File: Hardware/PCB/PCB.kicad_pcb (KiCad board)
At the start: 2 copper layers, 50.2 x 30.8 mm, 3 parts, among them P1 USB_C_Plug_USB2.0, U1 ESP32-H2-MINI-1, U3 AMS1117-3.3

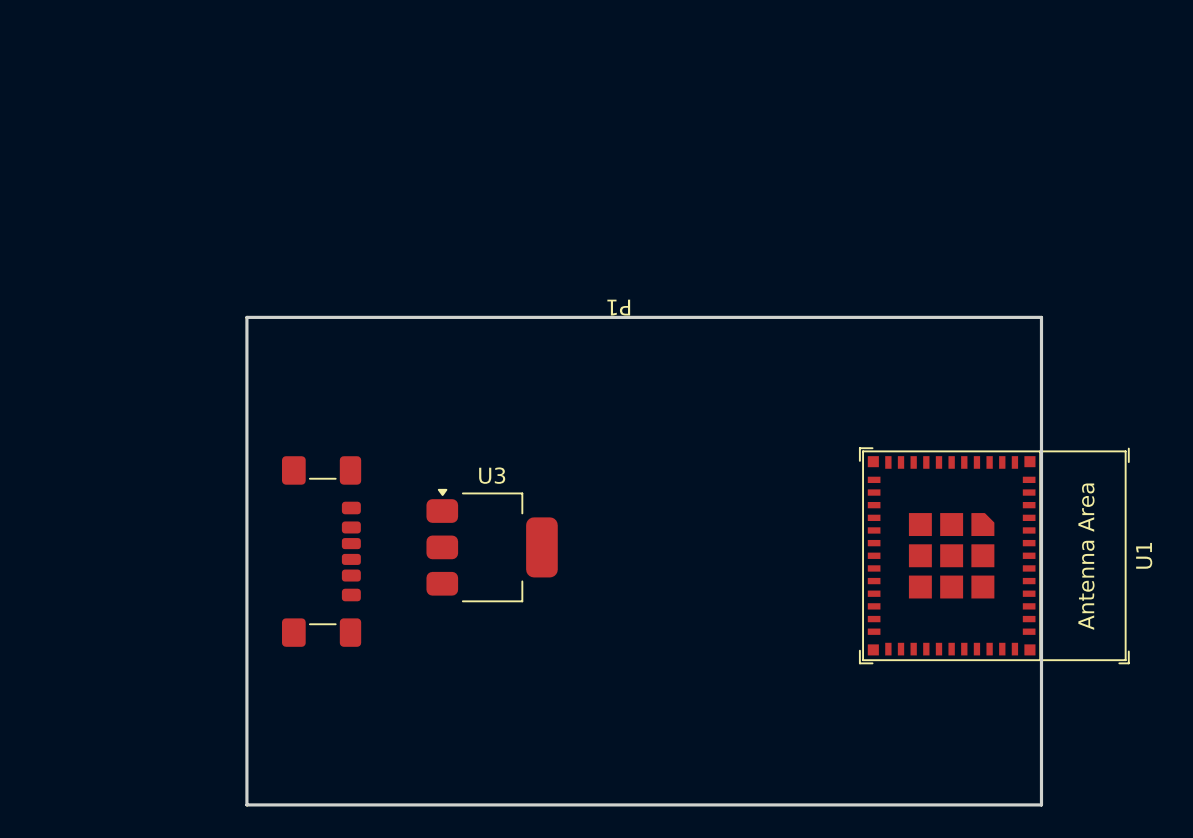
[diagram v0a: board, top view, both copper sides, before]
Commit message: First pass at full layout
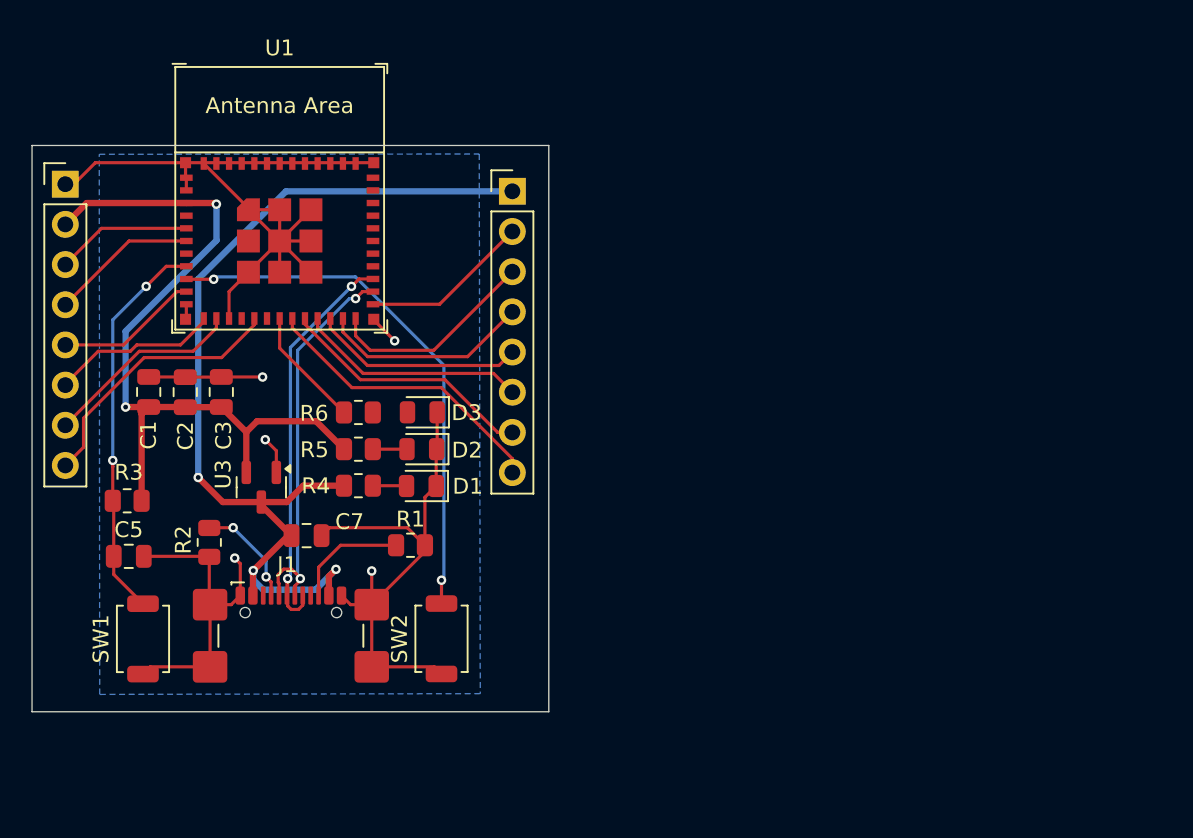
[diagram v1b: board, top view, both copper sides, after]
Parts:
- removed P1: USB_C_Plug_USB2.0, Connector_USB:USB_C_Receptacle_GCT_USB4135-GF-A_6P_TopMnt_Horizontal
- added C1: 10µ, Capacitor_SMD:C_0805_2012Metric, F.Cu at (97.3, 54.6)
- added C2: 1µF, Capacitor_SMD:C_0805_2012Metric, F.Cu at (99.6, 54.6)
- added C3: 0.1µ, Capacitor_SMD:C_0805_2012Metric, F.Cu at (101.9, 54.6)
- added C5: 1µ, Capacitor_SMD:C_0805_2012Metric, F.Cu at (96.0, 65.0)
- added C7: 1µF, Capacitor_SMD:C_0805_2012Metric, F.Cu at (107.3, 63.7)
- added D1: LED, LED_SMD:LED_0805_2012Metric, F.Cu at (114.5, 60.6)
- added D2: LED, LED_SMD:LED_0805_2012Metric, F.Cu at (114.6, 58.2)
- added D3: LED, LED_SMD:LED_0805_2012Metric, F.Cu at (114.6, 55.9)
- added J1: USB_C_Receptacle_USB2.0_14P, Connector_USB:USB_C_Receptacle_GCT_USB4110, F.Cu at (106.3, 71.2)
- added J2: Conn_01x08_Pin, Connector_PinHeader_2.54mm:PinHeader_1x08_P2.54mm_Vertical, F.Cu at (92.0, 41.5)
- added J3: Conn_01x8_Pin, Connector_PinHeader_2.54mm:PinHeader_1x08_P2.54mm_Vertical, F.Cu at (120.3, 41.9)
- added R1: 5.1K, Resistor_SMD:R_0805_2012Metric, F.Cu at (113.8, 64.3)
- added R2: 5.1K, Resistor_SMD:R_0805_2012Metric, F.Cu at (101.1, 64.1)
- added R3: 10K, Resistor_SMD:R_0805_2012Metric, F.Cu at (95.9, 61.5)
- added R4: 5.1K, Resistor_SMD:R_0805_2012Metric, F.Cu at (110.6, 60.5)
- added R5: 5.1K, Resistor_SMD:R_0805_2012Metric, F.Cu at (110.6, 58.2)
- added R6: 5.1K, Resistor_SMD:R_0805_2012Metric, F.Cu at (110.6, 55.9)
- added SW1: SW_Push, Button_Switch_SMD:SW_SPST_TS-1088-xR025, F.Cu at (96.9, 70.2)
- added SW2: SW_Push, Button_Switch_SMD:SW_SPST_TS-1088-xR025, F.Cu at (115.8, 70.2)
- U3: value AMS1117-3.3 -> MCP1700x-330xxTT; footprint Package_TO_SOT_SMD:SOT-223-3_TabPin2 -> Package_TO_SOT_SMD:SOT-23
- moved U1 50.5 mm to (105.6, 42.4), turned to 0 degrees
- moved U3 15.1 mm to (104.4, 60.6), turned to -90 degrees
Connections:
- net Net-(U1-3V3) renamed +3.3V
- U1 pad 10: unconnected-(U1-GPIO1/FSPICS0/ADC1_CH0-Pad10) -> GPIO1
- U1 pad 12: unconnected-(U1-GPIO13/XTAL_32K_P-Pad12) -> GPIO13
- U1 pad 13: unconnected-(U1-GPIO14/XTAL_32K_N-Pad13) -> GPIO14
- U1 pad 16: unconnected-(U1-GPIO12-Pad16) -> GPIO12
- U1 pad 18: unconnected-(U1-GPIO4/FSPICLK/ADC1_CH3/MTCK-Pad18) -> GPIO4
- U1 pad 19: unconnected-(U1-GPIO5/FSPID/ADC1_CH4/MTDI-Pad19) -> GPIO5
- U1 pad 20: unconnected-(U1-GPIO10/ZCD0-Pad20) -> GPIO10
- U1 pad 21: unconnected-(U1-GPIO11/ZCD1-Pad21) -> GPIO11
- U1 pad 22: unconnected-(U1-GPIO8-Pad22) -> GPIO8
- U1 pad 23: unconnected-(U1-GPIO9-Pad23) -> GPIO9
- U1 pad 24: unconnected-(U1-GPIO22-Pad24) -> GPIO22
- U1 pad 25: unconnected-(U1-GPIO25/FSPICS3-Pad25) -> GPIO25
- U1 pad 26: /USB_D- -> USB_D-
- U1 pad 27: /USB_D+ -> USB_D+
- U1 pad 30: unconnected-(U1-GPIO23/FSPICS1/U0RXD-Pad30) -> GPIO23
- U1 pad 31: unconnected-(U1-GPIO24/FSPICS2/U0TXD-Pad31) -> GPIO24
- U1 pad 5: unconnected-(U1-GPIO2/FSPIWP/ADC1_CH1/MTMS-Pad5) -> GPIO2
- U1 pad 6: unconnected-(U1-GPIO3/FSPIHD/ADC1_CH2/MTDO-Pad6) -> GPIO3
- U1 pad 8: unconnected-(U1-EN-Pad8) -> EN
- U1 pad 9: unconnected-(U1-GPIO0/FSPIQ-Pad9) -> BOOT
- U3 pad 3: Net-(U3-VI) -> +5V
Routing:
- net GND: track 0.00 -> 114.8 mm, vias 0 -> 5
- net +5V: track 0.00 -> 61.2 mm, vias 0 -> 3
- net +3.3V: track 0.00 -> 49.5 mm, vias 0 -> 2
- net BOOT: track 0.00 -> 33.8 mm, vias 0 -> 2
- net USB_D+: track 0.00 -> 26.3 mm, vias 0 -> 2
- net USB_D-: track 0.00 -> 25.2 mm, vias 0 -> 2
- net EN: track 0.00 -> 24.8 mm, vias 0 -> 2
- net GPIO5: track 0.00 -> 18.8 mm
- net GPIO12: track 0.00 -> 17.1 mm
- net GPIO10: track 0.00 -> 16.3 mm
- net GPIO11: track 0.00 -> 14.6 mm
- net GPIO8: track 0.00 -> 13.5 mm
- net GPIO22: track 0.00 -> 13.4 mm
- net GPIO9: track 0.00 -> 13.4 mm
- net GPIO14: track 0.00 -> 12.7 mm
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- added copper zone on B.Cu, net GND
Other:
- board size 50.2 x 30.8 mm -> 32.7 x 35.8 mm
